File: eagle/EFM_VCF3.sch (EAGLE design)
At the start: 21 parts, among them IC1 LM13700N, Q3 2N3906, Q4 2N3906, U1 POWER

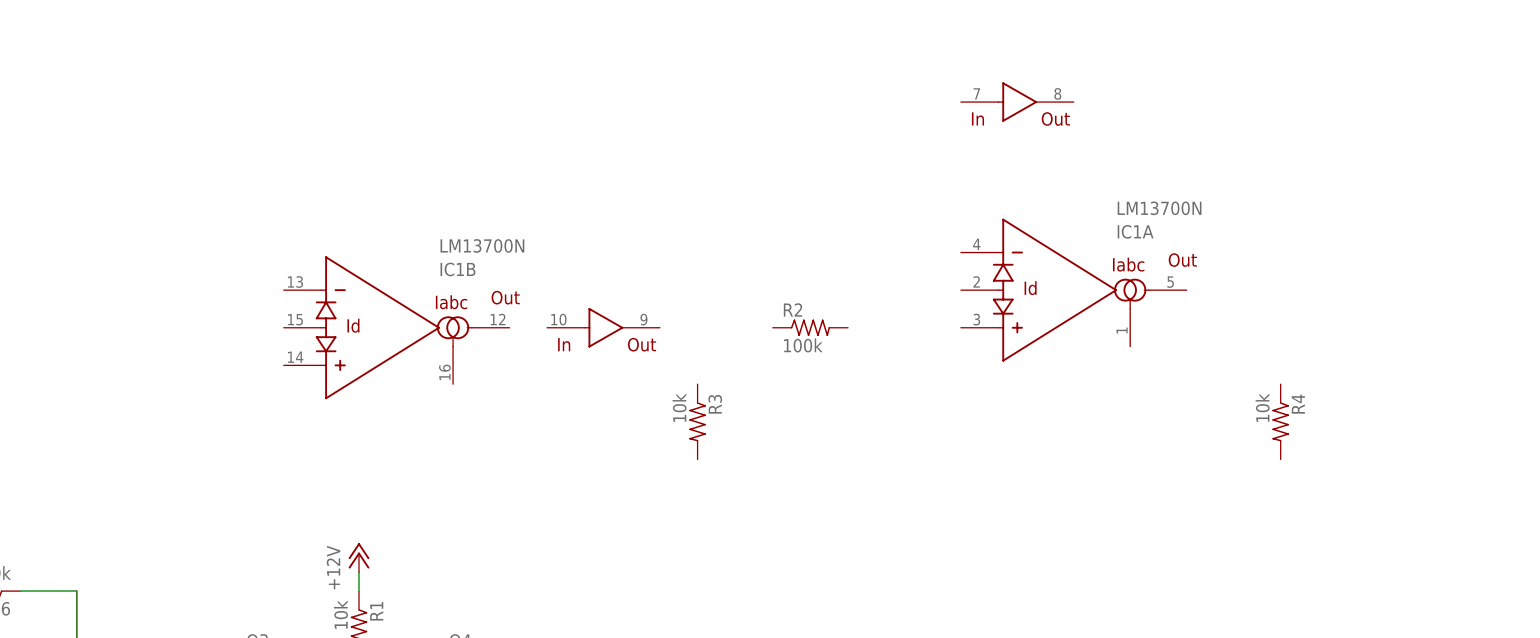
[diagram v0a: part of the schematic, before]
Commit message: more parts
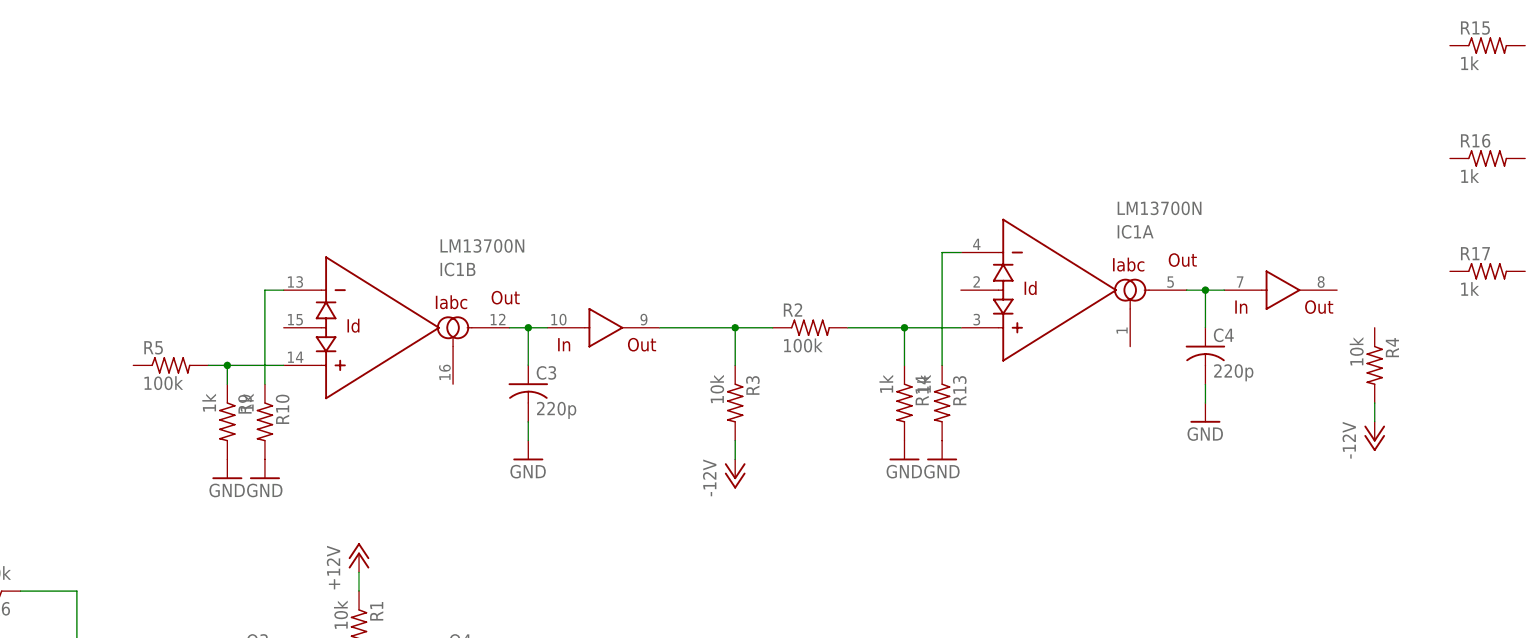
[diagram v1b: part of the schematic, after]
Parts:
- added C3, C4: 220p, rcl:C-US075-032X103
- added R10, R13, R14, R15, R16, R17, R9: 1k, rcl:R-US_0207/7
- added R5: 100k, rcl:R-US_0207/7
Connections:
- new net N$2: C3.1, IC1B.OUT, IC1G$4.IN
- new net N$3: C4.1, IC1A.OUT, IC1G$3.IN
- new net N$4: IC1B.+IN, R5.2, R9.1
- new net N$5: IC1G$4.OUT, R2.1, R3.1
- new net N$6: IC1A.+IN, R14.1, R2.2
- new net N$7: IC1B.-IN, R10.1
- new net N$8: IC1A.-IN, R13.1
- net -12V: now also R3.2, R4.2
- net GND: now also C3.2, C4.2, R10.2, R13.2, R14.2, R9.2
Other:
- moved on the sheet: R3, R4
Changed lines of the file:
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@@
 <part name="R3" library="rcl" deviceset="R-US_" device="0207/7" value="10k"/>
 <part name="R4" library="rcl" deviceset="R-US_" device="0207/7" value="10k"/>
+<part name="C3" library="rcl" deviceset="C-US" device="075-032X103" value="220p"/>
+<part name="C4" library="rcl" deviceset="C-US" device="075-032X103" value="220p"/>
+<part name="GND3" library="supply1" deviceset="GND" device=""/>
+<part name="GND6" library="supply1" deviceset="GND" device=""/>
+<part name="P-5" library="supply1" deviceset="-12V" device=""/>
+<part name="P-6" library="supply1" deviceset="-12V" device=""/>
+<part name="R5" library="rcl" deviceset="R-US_" device="0207/7" value="100k"/>
+<part name="R9" library="rcl" deviceset="R-US_" device="0207/7" value="1k"/>
+<part name="R10" library="rcl" deviceset="R-US_" device="0207/7" value="1k"/>
+<part name="R13" library="rcl" deviceset="R-US_" device="0207/7" value="1k"/>
+<part name="R14" library="rcl" deviceset="R-US_" device="0207/7" value="1k"/>
+<part name="GND7" library="supply1" deviceset="GND" device=""/>
+<part name="GND8" library="supply1" deviceset="GND" device=""/>
+<part name="GND11" library="supply1" deviceset="GND" device=""/>
+<part name="GND12" library="supply1" deviceset="GND" device=""/>
+<part name="R15" library="rcl" deviceset="R-US_" device="0207/7" value="1k"/>
+<part name="R16" library="rcl" deviceset="R-US_" device="0207/7" value="1k"/>
+<part name="R17" library="rcl" deviceset="R-US_" device="0207/7" value="1k"/>
 </parts>
 <sheets>
@@
 <instances>
 <instance part="IC1" gate="A" x="86.36" y="109.22"/>
-<instance part="IC1" gate="G$3" x="83.82" y="134.62"/>
+<instance part="IC1" gate="G$3" x="119.38" y="109.22"/>
 <instance part="IC1" gate="G$4" x="27.94" y="104.14"/>
 <instance part="IC1" gate="B" x="-5.08" y="104.14"/>
@@
 <instance part="P+6" gate="1" x="-5.08" y="73.66"/>
 <instance part="R2" gate="G$1" x="55.88" y="104.14"/>
-<instance part="R3" gate="G$1" x="40.64" y="91.44" rot="R270"/>
-<instance part="R4" gate="G$1" x="119.38" y="91.44" rot="R270"/>
+<instance part="R3" gate="G$1" x="45.72" y="93.98" rot="R270"/>
+<instance part="R4" gate="G$1" x="132.08" y="99.06" rot="R270"/>
+<instance part="C3" gate="G$1" x="17.78" y="96.52"/>
+<instance part="C4" gate="G$1" x="109.22" y="101.6"/>
+<instance part="GND3" gate="1" x="17.78" y="86.36"/>
+<instance part="GND6" gate="1" x="109.22" y="91.44"/>
+<instance part="P-5" gate="1" x="45.72" y="83.82"/>
+<instance part="P-6" gate="1" x="132.08" y="88.9"/>
+<instance part="R5" gate="G$1" x="-30.48" y="99.06"/>
+<instance part="R9" gate="G$1" x="-22.86" y="91.44" rot="R270"/>
+<instance part="R10" gate="G$1" x="-17.78" y="91.44" rot="R270"/>
+<instance part="R13" gate="G$1" x="73.66" y="93.98" rot="R270"/>
+<instance part="R14" gate="G$1" x="68.58" y="93.98" rot="R270"/>
+<instance part="GND7" gate="1" x="68.58" y="86.36"/>
+<instance part="GND8" gate="1" x="73.66" y="86.36"/>
+<instance part="GND11" gate="1" x="-17.78" y="83.82"/>
+<instance part="GND12" gate="1" x="-22.86" y="83.82"/>
+<instance part="R15" gate="G$1" x="147.32" y="142.24"/>
+<instance part="R16" gate="G$1" x="147.32" y="127"/>
+<instance part="R17" gate="G$1" x="147.32" y="111.76"/>
 </instances>
 <busses>
@@
 <pinref part="GND9" gate="1" pin="GND"/>
 </segment>
+<segment>
+<pinref part="C3" gate="G$1" pin="2"/>
+<pinref part="GND3" gate="1" pin="GND"/>
+<wire x1="17.78" y1="91.44" x2="17.78" y2="88.9" width="0.1524" layer="91"/>
+</segment>
+<segment>
+<pinref part="C4" gate="G$1" pin="2"/>
+<pinref part="GND6" gate="1" pin="GND"/>
+<wire x1="109.22" y1="93.98" x2="109.22" y2="96.52" width="0.1524" layer="91"/>
+</segment>
+<segment>
+<pinref part="R14" gate="G$1" pin="2"/>
+<pinref part="GND7" gate="1" pin="GND"/>
+</segment>
+<segment>
+<pinref part="R13" gate="G$1" pin="2"/>
+<pinref part="GND8" gate="1" pin="GND"/>
+</segment>
+<segment>
+<pinref part="R10" gate="G$1" pin="2"/>
+<pinref part="GND11" gate="1" pin="GND"/>
+</segment>
+<segment>
+<pinref part="R9" gate="G$1" pin="2"/>
+<pinref part="GND12" gate="1" pin="GND"/>
+</segment>
 </net>
 <net name="N$38" class="0">
@@
 <wire x1="66.04" y1="27.94" x2="66.04" y2="24.384" width="0.1524" layer="91"/>
 <pinref part="C2" gate="G$1" pin="-"/>
+</segment>
+<segment>
+<pinref part="R3" gate="G$1" pin="2"/>
+<pinref part="P-5" gate="1" pin="-12V"/>
+<wire x1="45.72" y1="88.9" x2="45.72" y2="86.36" width="0.1524" layer="91"/>
+</segment>
+<segment>
+<pinref part="R4" gate="G$1" pin="2"/>
+<pinref part="P-6" gate="1" pin="-12V"/>
+<wire x1="132.08" y1="91.44" x2="132.08" y2="93.98" width="0.1524" layer="91"/>
 </segment>
 </net>
@@
 </segment>
 </net>
+<net name="N$2" class="0">
+<segment>
+<pinref part="IC1" gate="B" pin="OUT"/>
+<pinref part="IC1" gate="G$4" pin="IN"/>
+<wire x1="20.32" y1="104.14" x2="17.78" y2="104.14" width="0.1524" layer="91"/>
+<pinref part="C3" gate="G$1" pin="1"/>
+<wire x1="17.78" y1="104.14" x2="15.24" y2="104.14" width="0.1524" layer="91"/>
+<wire x1="17.78" y1="99.06" x2="17.78" y2="104.14" width="0.1524" layer="91"/>
+<junction x="17.78" y="104.14"/>
+</segment>
+</net>
+<net name="N$3" class="0">
+<segment>
+<pinref part="IC1" gate="A" pin="OUT"/>
+<pinref part="IC1" gate="G$3" pin="IN"/>
+<wire x1="111.76" y1="109.22" x2="109.22" y2="109.22" width="0.1524" layer="91"/>
+<pinref part="C4" gate="G$1" pin="1"/>
+<wire x1="109.22" y1="109.22" x2="106.68" y2="109.22" width="0.1524" layer="91"/>
+<wire x1="109.22" y1="104.14" x2="109.22" y2="109.22" width="0.1524" layer="91"/>
+<junction x="109.22" y="109.22"/>
+</segment>
+</net>
+<net name="N$4" class="0">
+<segment>
+<pinref part="IC1" gate="B" pin="+IN"/>
+<pinref part="R5" gate="G$1" pin="2"/>
+<wire x1="-25.4" y1="99.06" x2="-22.86" y2="99.06" width="0.1524" layer="91"/>
+<pinref part="R9" gate="G$1" pin="1"/>
+<wire x1="-22.86" y1="99.06" x2="-15.24" y2="99.06" width="0.1524" layer="91"/>
+<wire x1="-22.86" y1="96.52" x2="-22.86" y2="99.06" width="0.1524" layer="91"/>
+<junction x="-22.86" y="99.06"/>
+</segment>
+</net>
+<net name="N$5" class="0">
+<segment>
+<pinref part="IC1" gate="G$4" pin="OUT"/>
+<pinref part="R2" gate="G$1" pin="1"/>
+<wire x1="50.8" y1="104.14" x2="45.72" y2="104.14" width="0.1524" layer="91"/>
+<pinref part="R3" gate="G$1" pin="1"/>
+<wire x1="45.72" y1="104.14" x2="35.56" y2="104.14" width="0.1524" layer="91"/>
+<wire x1="45.72" y1="99.06" x2="45.72" y2="104.14" width="0.1524" layer="91"/>
+<junction x="45.72" y="104.14"/>
+</segment>
+</net>
+<net name="N$6" class="0">
+<segment>
+<pinref part="IC1" gate="A" pin="+IN"/>
+<pinref part="R2" gate="G$1" pin="2"/>
+<wire x1="60.96" y1="104.14" x2="68.58" y2="104.14" width="0.1524" layer="91"/>
+<pinref part="R14" gate="G$1" pin="1"/>
+<wire x1="68.58" y1="104.14" x2="76.2" y2="104.14" width="0.1524" layer="91"/>
+<wire x1="68.58" y1="99.06" x2="68.58" y2="104.14" width="0.1524" layer="91"/>
+<junction x="68.58" y="104.14"/>
+</segment>
+</net>
+<net name="N$7" class="0">
+<segment>
+<pinref part="R10" gate="G$1" pin="1"/>
+<wire x1="-17.78" y1="96.52" x2="-17.78" y2="109.22" width="0.1524" layer="91"/>
+<pinref part="IC1" gate="B" pin="-IN"/>
+<wire x1="-17.78" y1="109.22" x2="-15.24" y2="109.22" width="0.1524" layer="91"/>
+</segment>
+</net>
+<net name="N$8" class="0">
+<segment>
+<pinref part="IC1" gate="A" pin="-IN"/>
+<pinref part="R13" gate="G$1" pin="1"/>
+<wire x1="76.2" y1="114.3" x2="73.66" y2="114.3" width="0.1524" layer="91"/>
+<wire x1="73.66" y1="114.3" x2="73.66" y2="99.06" width="0.1524" layer="91"/>
+</segment>
+</net>
